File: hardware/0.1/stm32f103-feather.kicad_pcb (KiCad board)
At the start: 2 copper layers, 51.8 x 22.9 mm, 41 parts, among them J1 1.27_SWD, J2 USB_C_Receptacle_USB2.0, J3 JST_PH, J4 Feather, Q1 DMP2045U, SW1 SW_Push, SW2 SW_Push, U1 STM32F103C8Tx, U2 AP2112K-3.3, U3 MCP73831-2-OT, Y1 8MHz

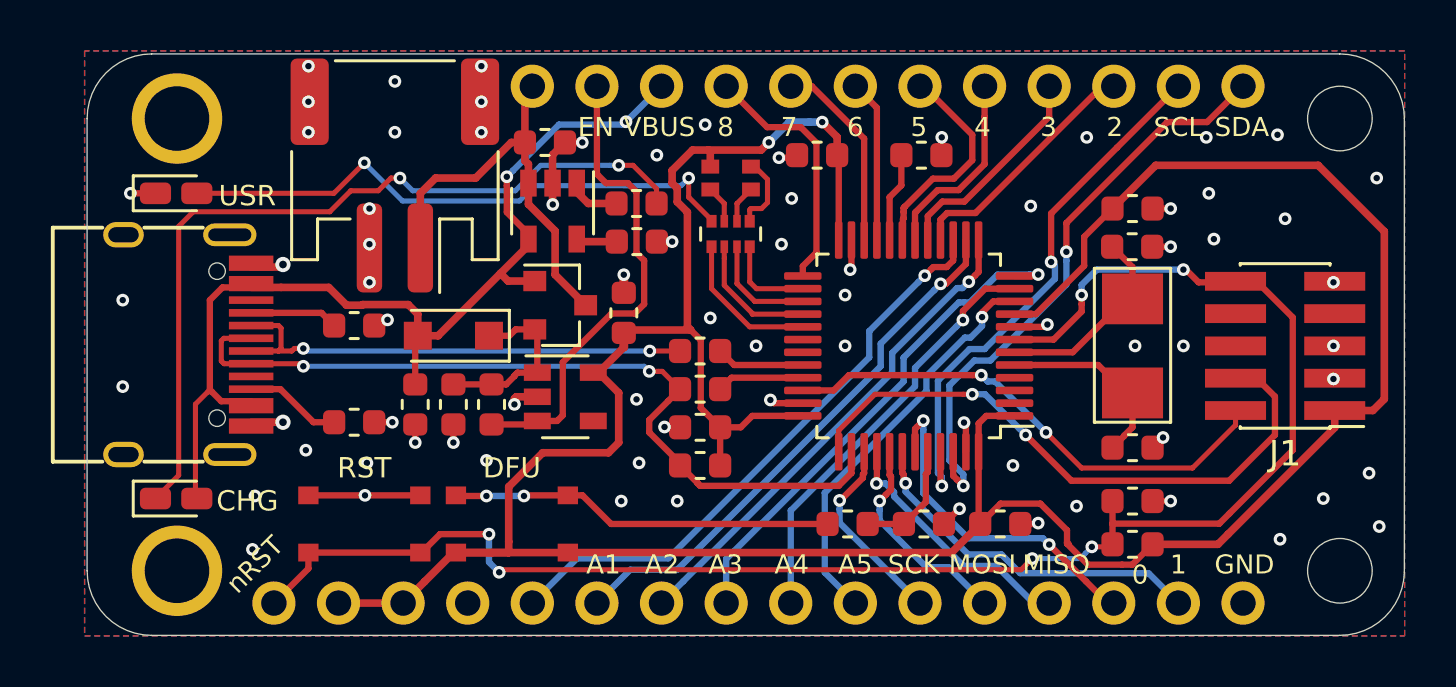
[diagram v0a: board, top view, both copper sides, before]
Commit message: change osc footprint
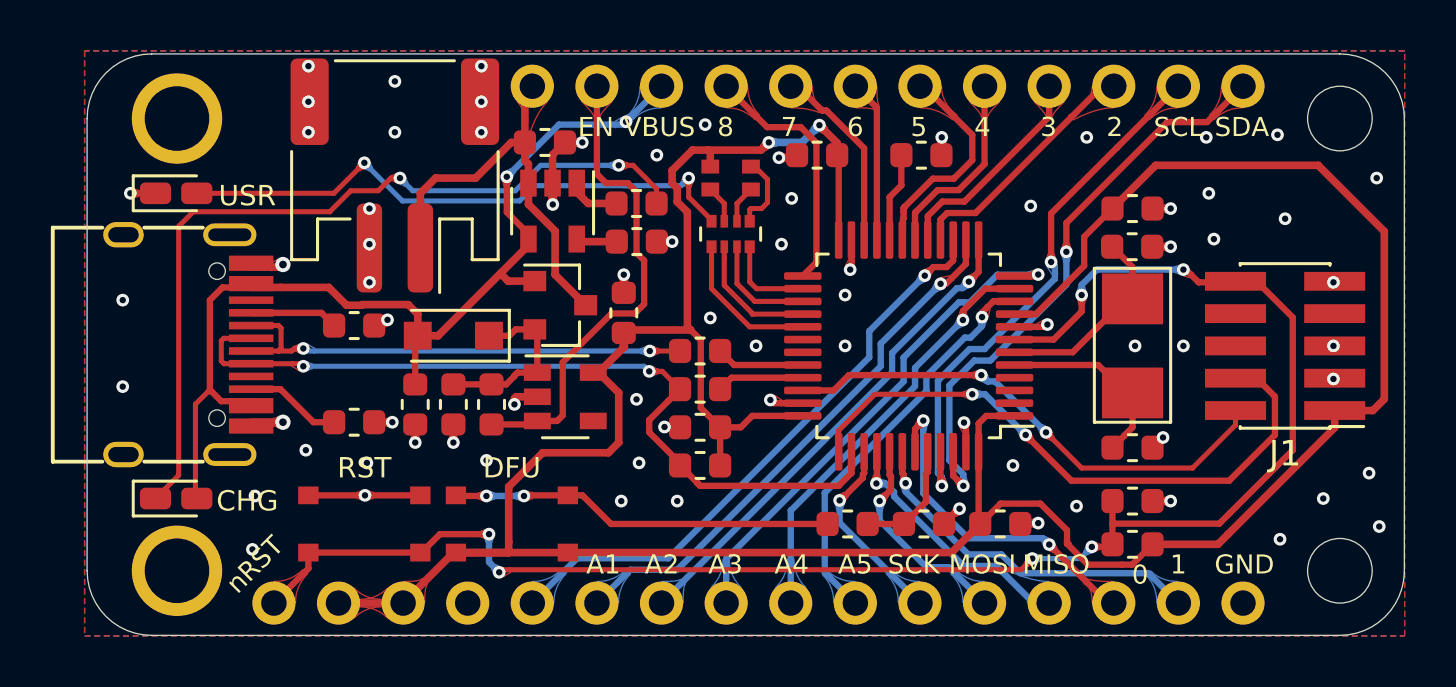
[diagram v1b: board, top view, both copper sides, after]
